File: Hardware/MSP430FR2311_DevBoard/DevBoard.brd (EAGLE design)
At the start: 25 x 22 mm, 27 parts, among them IC1 MSP430FR2311IPW20, IC2 TLV75801PDRVT, Y1 ABS05-32.768KHZ-9-T

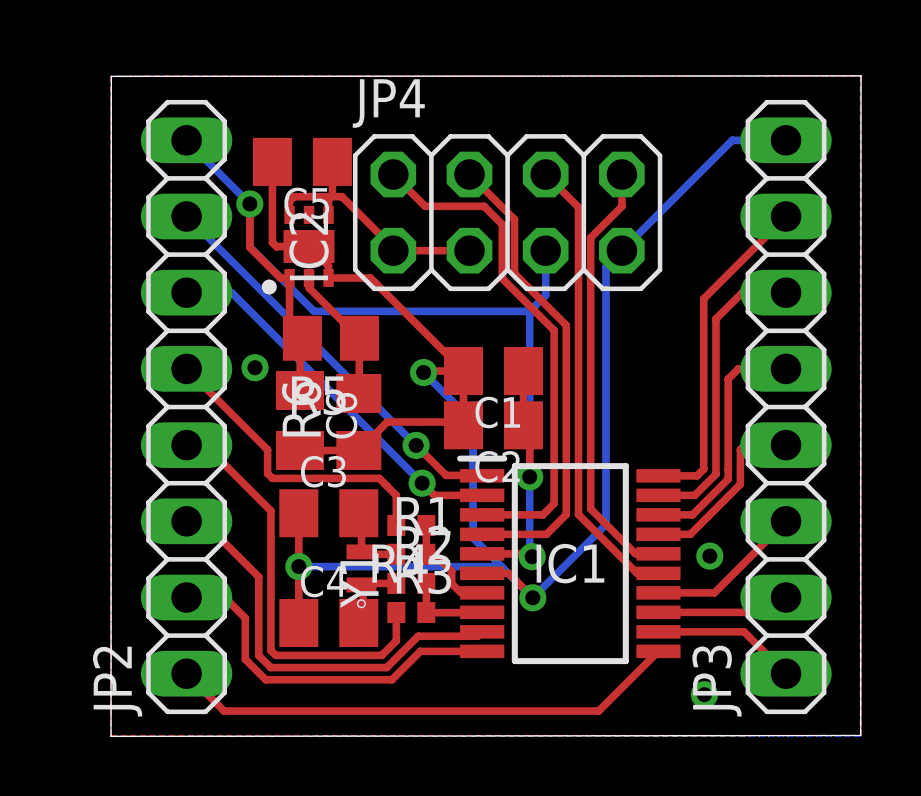
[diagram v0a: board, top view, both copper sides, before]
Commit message: hardware updates
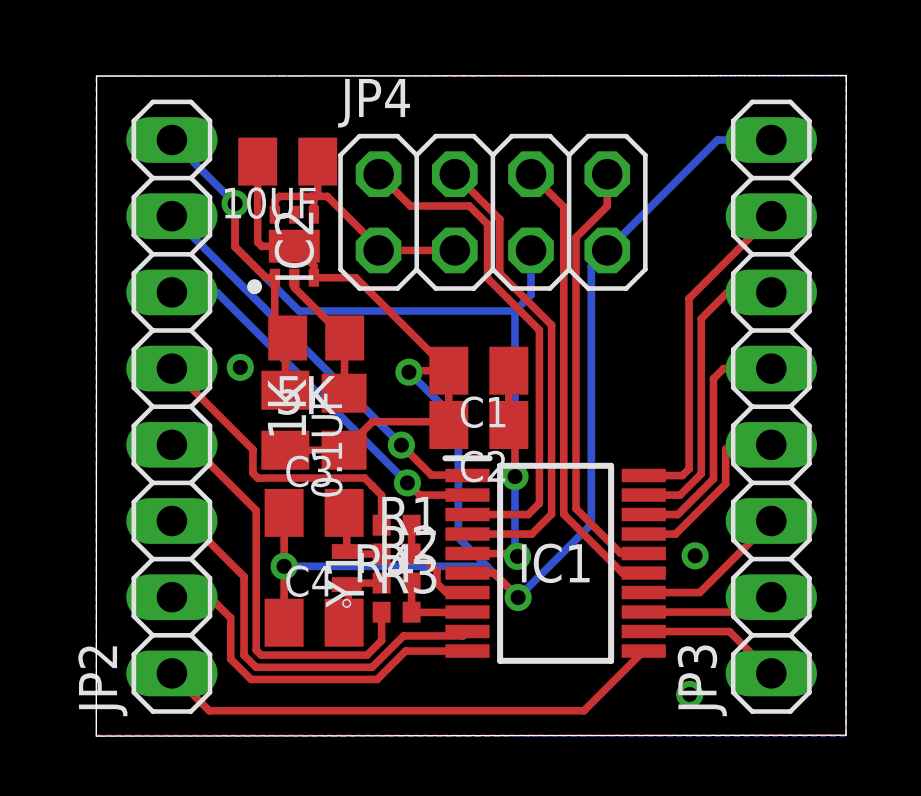
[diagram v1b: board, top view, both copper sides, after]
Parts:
- removed C5, C6: (no value), rcl:C0805K
- removed R5, R6: (no value), rcl:R0805
- removed U$6: (no value), ruler:METRIC_15
- added 0.1UF, 10UF: (no value), rcl:C0805K
- added 1K, 5K: (no value), rcl:R0805
- moved C2 0.49 mm to (12.8, 10.4)
- moved C1 0.49 mm to (12.8, 12.2)
- moved C3 0.49 mm to (7.27, 7.45)
- moved C4 0.49 mm to (7.27, 3.79)
- moved IC1 0.49 mm to (15.3, 5.77)
- moved JP2 0.49 mm to (2.53, 11.0)
- moved JP4 0.49 mm to (13.2, 17.5)
- moved R1 0.49 mm to (10.0, 6.08)
- moved R2 0.49 mm to (10.0, 5.11)
- moved R3 0.49 mm to (10.0, 4.14)
- moved R4 0.49 mm to (10.0, 7.04)
- moved U$7 0.49 mm to (2.50, 0.02)
- moved U$8 0.49 mm to (12.0, 0.02)
- moved Y1 0.49 mm to (8.36, 5.61)
- moved U$4 0.49 mm to (0.02, 22.0)
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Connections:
- net +3V3: now also 0.1UF.1, 5K.2; no longer C6.1, R5.2
- net +5V: now also 10UF.1; no longer C5.1
- net GND: now also 0.1UF.2, 10UF.2, 1K.1; no longer C5.2, C6.2, R6.1
- net N$12: now also 1K.2, 5K.1; no longer R5.1, R6.2
